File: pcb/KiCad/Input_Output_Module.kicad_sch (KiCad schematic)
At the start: 52 parts, among them J11 Curr_In (Out2), J12 Error_In, J13 Curr_Out (Out2), J14 Error_Out (In1), J16 Error_Mon, J3 Piezo_In (Out1), J5 Piezo_Out, J7 Piezo_Monitor, U4 OPA1604, U5 BUF634, U7 OPA1602, U8 OPA1602

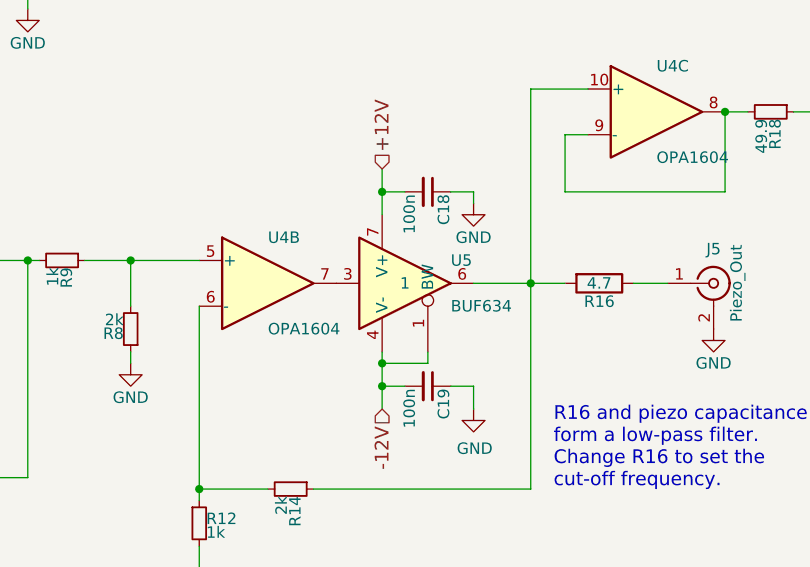
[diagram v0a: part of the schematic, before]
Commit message: Update BOM
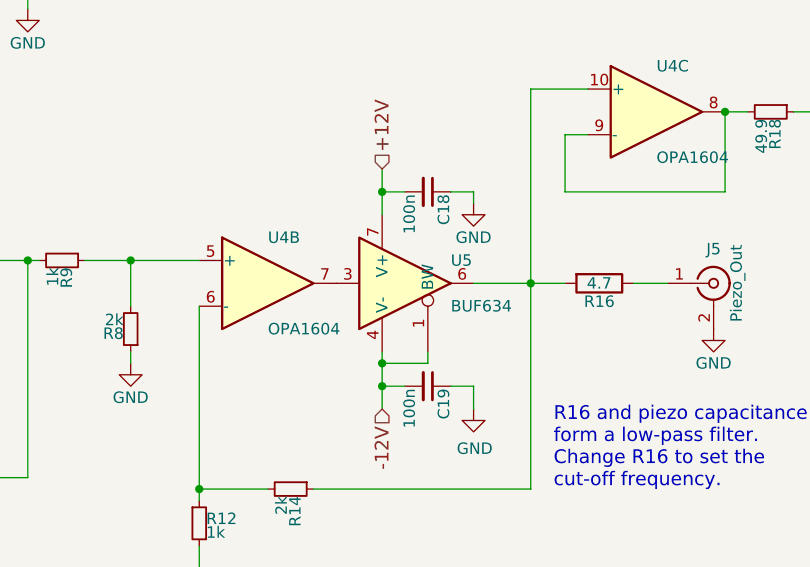
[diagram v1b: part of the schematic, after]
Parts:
- U5: Field4 1 -> (none)
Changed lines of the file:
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@@
       (effects (font (size 1.27 1.27)) hide)
     )
-    (property "Field4" "1" (id 6) (at 137.16 102.87 0))
     (pin "4")
     (pin "7")
